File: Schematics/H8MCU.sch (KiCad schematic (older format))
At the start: 4 parts

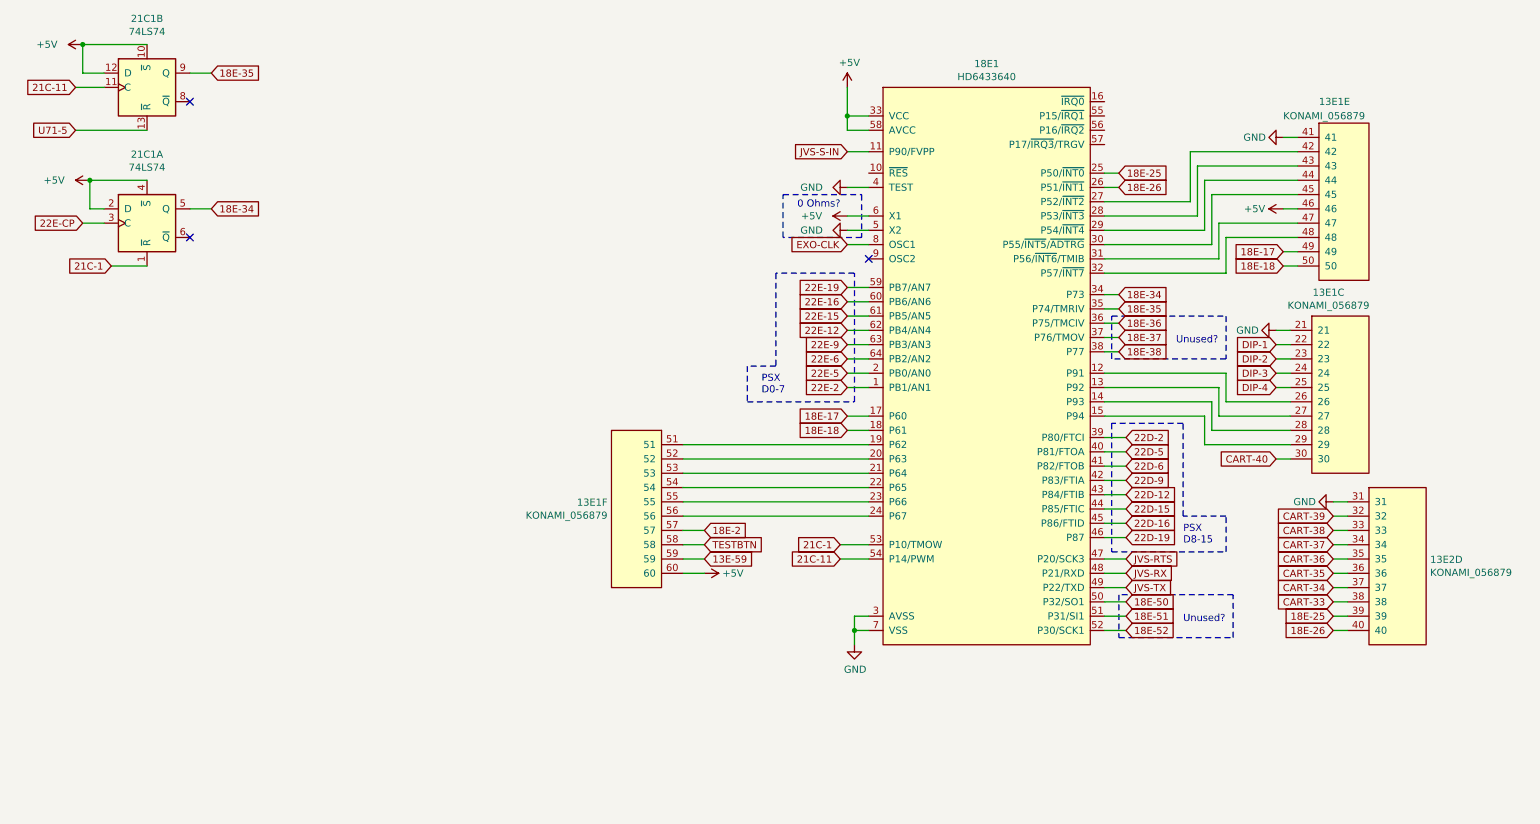
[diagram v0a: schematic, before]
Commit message: 573 specific mostly mapped
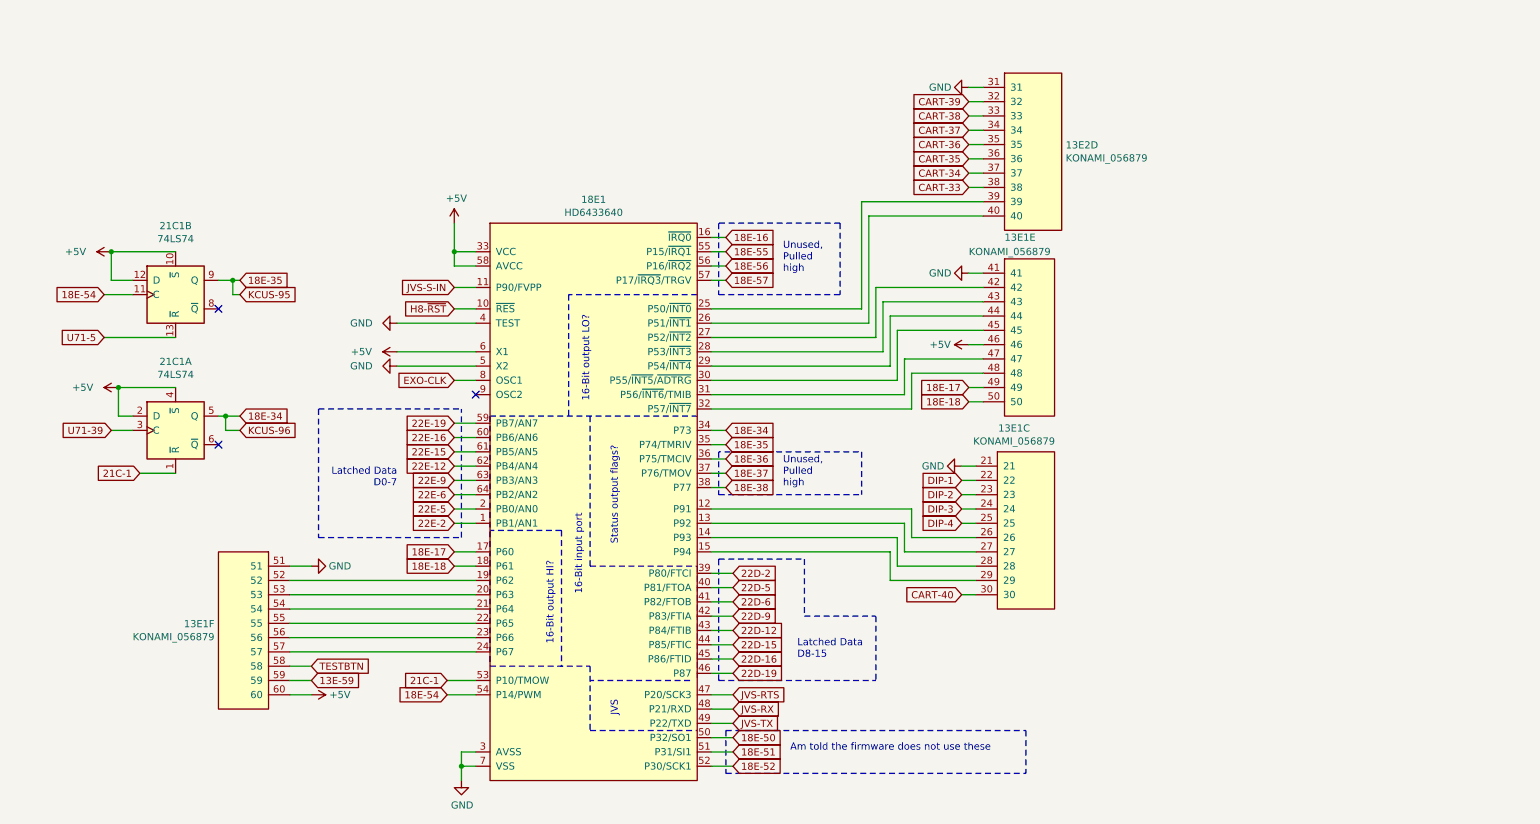
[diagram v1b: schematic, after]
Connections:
- net 18E-2 is gone; now on an unnamed net: 13E1.57
- net GND: now also 13E1.51
- net H8-~RST: now reaches 18E1.10 (~RES)
- net 18E-16: now reaches 18E1.16 (~IRQ0)
- net at 18E1.19 (P62): now also 13E1.52; no longer 13E1.51
- net at 18E1.20 (P63): now also 13E1.53; no longer 13E1.52
- net at 18E1.21 (P64): now also 13E1.54; no longer 13E1.53
- net at 18E1.22 (P65): now also 13E1.55; no longer 13E1.54
- net at 18E1.23 (P66): now also 13E1.56; no longer 13E1.55
- net at 18E1.24 (P67): no longer 13E1.56
- net 18E-55: now reaches 18E1.55 (P15/~IRQ1)
- net 18E-56: now reaches 18E1.56 (P16/~IRQ2)
- net 18E-57: now reaches 18E1.57 (P17/~IRQ3~/TRGV)
- net 18E-25: no longer names the net of 13E2.39, 18E1.25 (P50/~INT0)
- net 18E-26: no longer names the net of 13E2.40, 18E1.26 (P51/~INT1)
- net 21C-11 renamed 18E-54
- net 22E-CP renamed U71-39
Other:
- note added: "16-Bit input port"
- note added: "16-Bit output HI?"
- note added: "16-Bit output LO?"
- note added: "Am told the firmware does not use these"
- note added: "JVS"
- note added: "Latched Data\nD0-7"
- note added: "Latched Data\nD8-15"
- note added: "Status output flags?"
- note added: "Unused,\nPulled\nhigh"
- note removed: "0 Ohms?"
- note removed: "PSX\nD0-7"
- note removed: "PSX\nD8-15"
- note removed: "Unused?"
- moved on the sheet: 13E1C, 13E1E, 13E1F, 13E2D, 18E1, 21C1A, 21C1B
